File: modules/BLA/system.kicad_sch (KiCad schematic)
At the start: 2 parts, among them J2 CardConnector

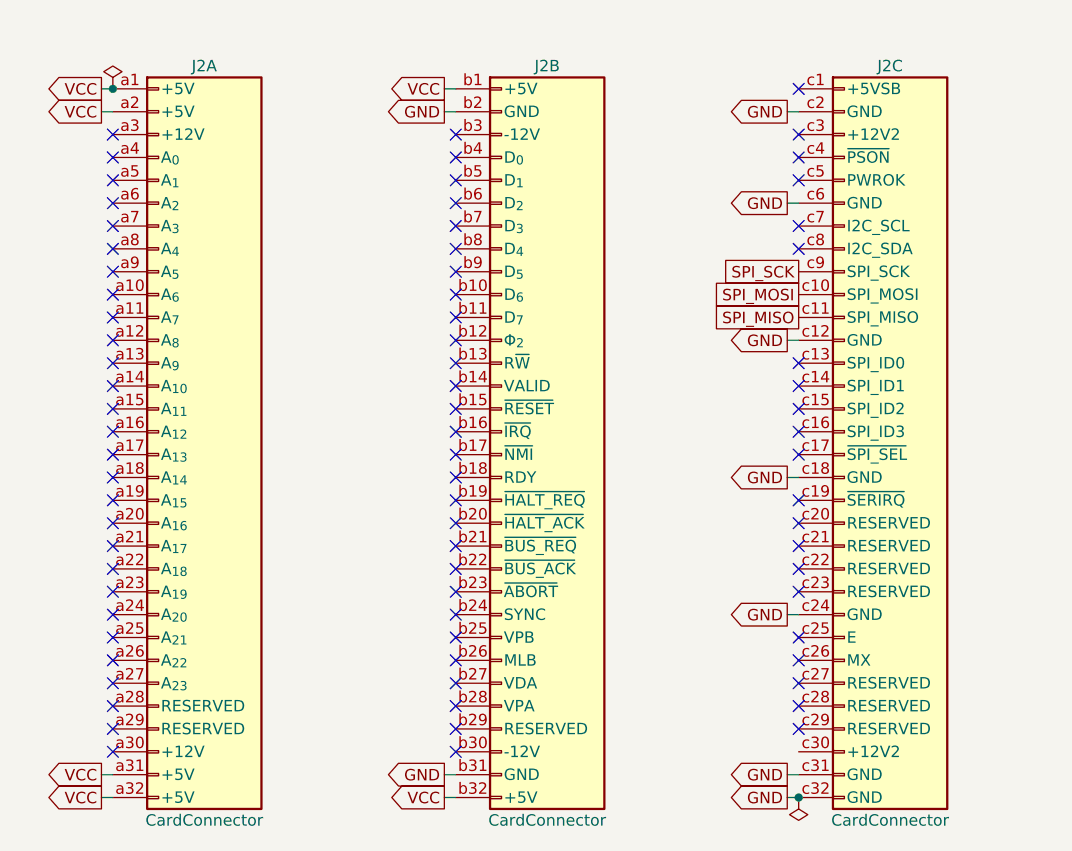
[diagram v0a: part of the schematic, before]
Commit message: minor PW PCB tweaks
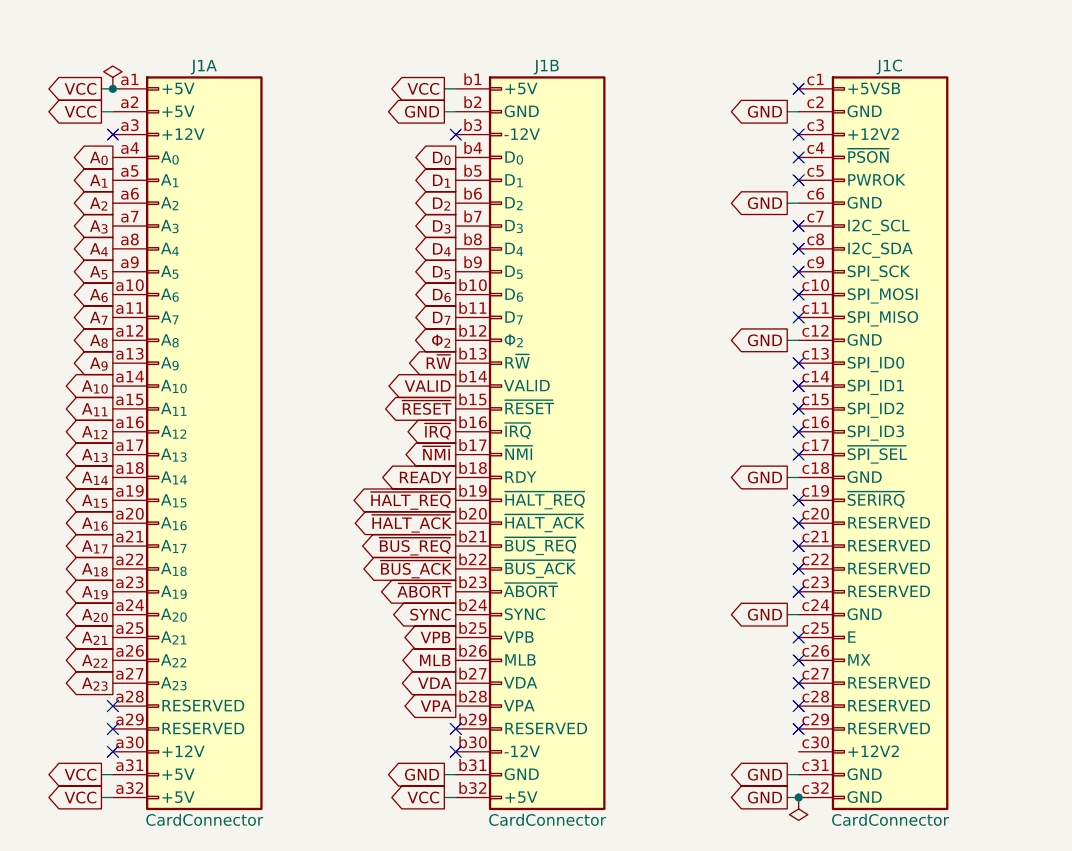
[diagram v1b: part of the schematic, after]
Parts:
- renumbered J2 to J1
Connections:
- net D_{6}: now reaches J1.b10 (D_{6})
- net D_{7}: now reaches J1.b11 (D_{7})
- net Φ_{2}: now reaches J1.b12 (Φ_{2})
- net R~{W}: now reaches J1.b13 (R~{W})
- net VALID: now reaches J1.b14 (VALID)
- net ~{RESET}: now reaches J1.b15 (~{RESET})
- net ~{IRQ}: now reaches J1.b16 (~{IRQ})
- net ~{NMI}: now reaches J1.b17 (~{NMI})
- net READY: now reaches J1.b18 (RDY)
- net ~{HALT_REQ}: now reaches J1.b19 (~{HALT_REQ})
- net ~{HALT_ACK}: now reaches J1.b20 (~{HALT_ACK})
- net ~{BUS_REQ}: now reaches J1.b21 (~{BUS_REQ})
- net ~{BUS_ACK}: now reaches J1.b22 (~{BUS_ACK})
- net ~{ABORT}: now reaches J1.b23 (~{ABORT})
- net SYNC: now reaches J1.b24 (SYNC)
- net VPB: now reaches J1.b25 (VPB)
- net MLB: now reaches J1.b26 (MLB)
- net VDA: now reaches J1.b27 (VDA)
- net VPA: now reaches J1.b28 (VPA)
- net D_{0}: now reaches J1.b4 (D_{0})
- net D_{1}: now reaches J1.b5 (D_{1})
- net D_{2}: now reaches J1.b6 (D_{2})
- net D_{3}: now reaches J1.b7 (D_{3})
- net D_{4}: now reaches J1.b8 (D_{4})
- net D_{5}: now reaches J1.b9 (D_{5})
- net A_{6}: now reaches J1.a10 (A_{6})
- net A_{7}: now reaches J1.a11 (A_{7})
- net A_{8}: now reaches J1.a12 (A_{8})
- net A_{9}: now reaches J1.a13 (A_{9})
- net A_{10}: now reaches J1.a14 (A_{10})
- net A_{11}: now reaches J1.a15 (A_{11})
- net A_{12}: now reaches J1.a16 (A_{12})
- net A_{13}: now reaches J1.a17 (A_{13})
- net A_{14}: now reaches J1.a18 (A_{14})
- net A_{15}: now reaches J1.a19 (A_{15})
- net A_{16}: now reaches J1.a20 (A_{16})
- net A_{17}: now reaches J1.a21 (A_{17})
- net A_{18}: now reaches J1.a22 (A_{18})
- net A_{19}: now reaches J1.a23 (A_{19})
- net A_{20}: now reaches J1.a24 (A_{20})
- net A_{21}: now reaches J1.a25 (A_{21})
- net A_{22}: now reaches J1.a26 (A_{22})
- net A_{23}: now reaches J1.a27 (A_{23})
- net A_{0}: now reaches J1.a4 (A_{0})
- net A_{1}: now reaches J1.a5 (A_{1})
- net A_{2}: now reaches J1.a6 (A_{2})
- net A_{3}: now reaches J1.a7 (A_{3})
- net A_{4}: now reaches J1.a8 (A_{4})
- net A_{5}: now reaches J1.a9 (A_{5})
- net SPI_MISO: no longer names the net of J1.c11 (SPI_MISO)
- net SPI_MOSI: no longer names the net of J1.c10 (SPI_MOSI)
- net SPI_SCK: no longer names the net of J1.c9 (SPI_SCK)
- no-connect marks 77 -> 31
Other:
- title: MSD-65 -> BLA-65

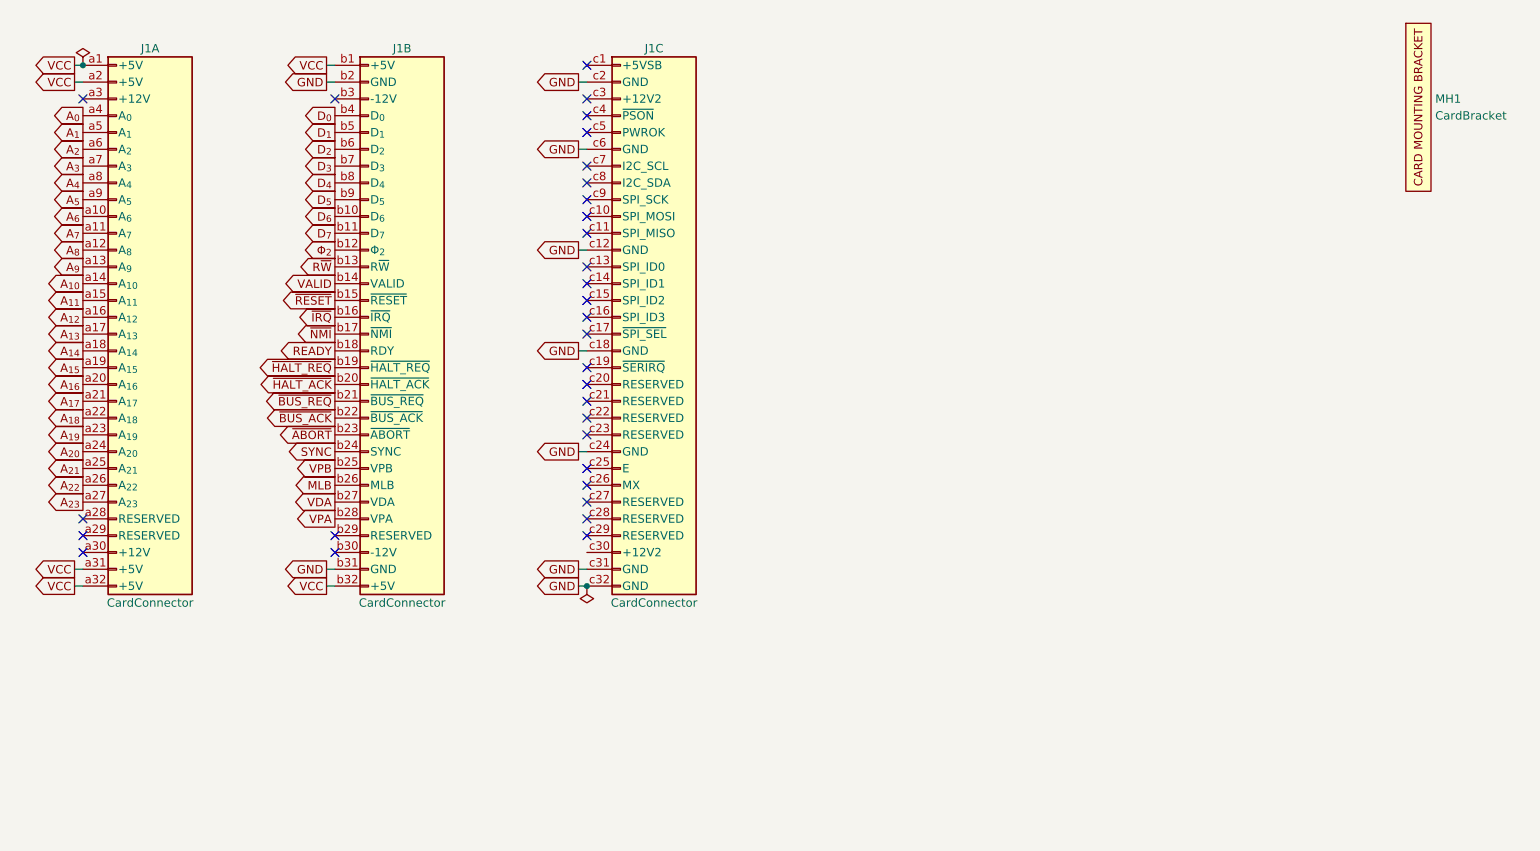
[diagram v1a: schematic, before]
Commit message: bla pcb and schematic
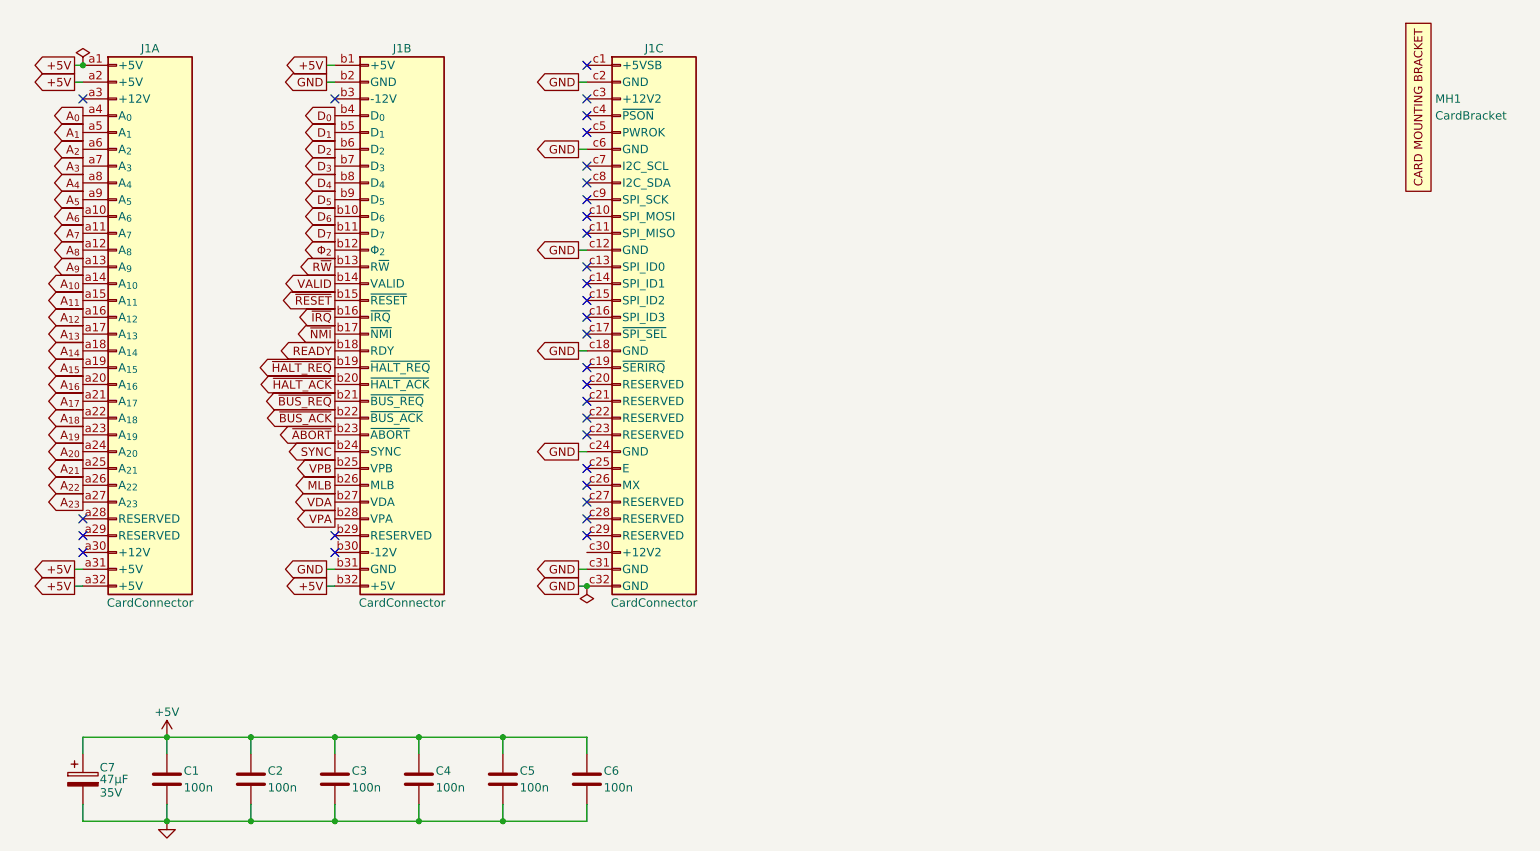
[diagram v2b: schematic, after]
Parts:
- added C1, C2, C3, C4, C5, C6: 100n, IMNOTWOPR:C_Rect_P200mil, symbol IMNOTWOPR:C
- added C7: 47µF, IMNOTWOPR:CP_Radial_Tantal_P100mil, symbol IMNOTWOPR:C_Polarized
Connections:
- net GND: now also C1.2, C2.2, C3.2, C4.2, C5.2, C6.2, C7.2
- net VCC renamed +5V
- net +5V: now also C1.1, C2.1, C3.1, C4.1, C5.1, C6.1, C7.1
